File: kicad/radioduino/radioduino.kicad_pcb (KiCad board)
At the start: 2 copper layers, 130.5 x 70 mm, 48 parts, among them J1 Conn_01x03_Socket, J2 Conn_Coaxial_Small, J3 Conn_Coaxial_Small, J4 Conn_Coaxial_Small, J5 Conn_Coaxial_Small, J6 Conn_01x15, J7 Conn_01x15, Q1 SS8050, Q2 BSS138, Q3 BSS138, SW1 RotaryEncoder_Switch_MP, U1 PCF8574AT, U2 RT9193-33GB, Y1 Si5351A-B-GT

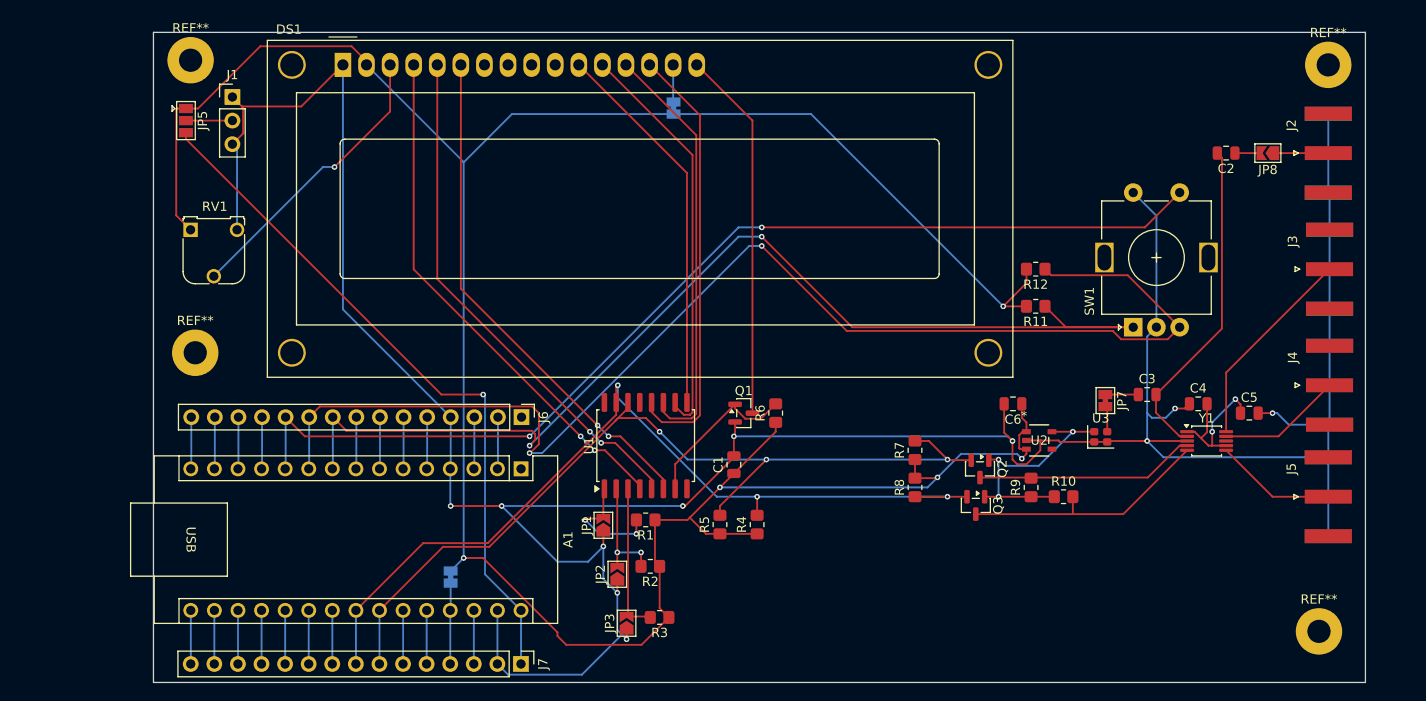
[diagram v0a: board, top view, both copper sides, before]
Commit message: pcb
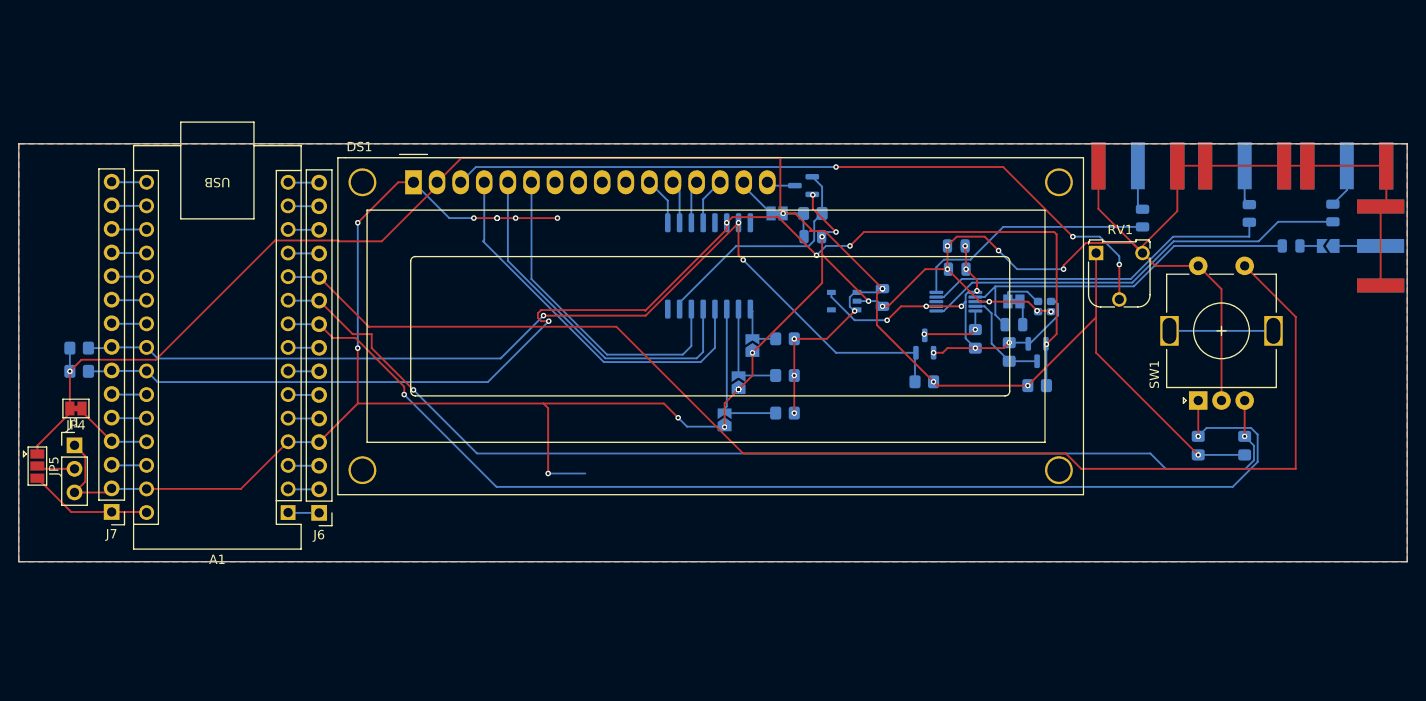
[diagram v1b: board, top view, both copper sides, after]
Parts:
- removed REF** (x4): MountingHole_2.5mm_Pad, MountingHole:MountingHole_2.5mm_Pad
- added C7: 100n, Capacitor_SMD:C_0805_2012Metric, B.Cu at (191.0, 65.0)
- added C8: 100n, Capacitor_SMD:C_0805_2012Metric, B.Cu at (202.5, 64.5)
- added C9: 100n, Capacitor_SMD:C_0805_2012Metric, B.Cu at (211.5, 64.5)
- C1, C2, C3, C4, C5, C6, J2, J3, J4, J5, JP1, JP2, JP3, JP7, JP8, Q1, Q2, Q3, R1, R10, R11, R12, R2, R3, R4, R5, R6, R7, R8, R9, U1, U2, U3, Y1: moved to B.Cu
- JP4: moved to F.Cu
- moved RV1 97.5 mm to (186.0, 68.8)
- moved R4 75.4 mm to (76.5, 79.0), turned to 0 degrees
- moved R5 70.9 mm to (76.5, 81.5), turned to 0 degrees
- moved J7 47.0 mm to (80.0, 96.6), turned to 180 degrees
- moved JP4 44.2 mm to (76.2, 85.5), turned to 180 degrees
- moved J1 41.2 mm to (76.0, 89.5)
- moved JP5 40.5 mm to (72.0, 91.7)
- moved C5 36.3 mm to (170.9, 68.0), turned to 180 degrees
- moved J5 35.7 mm to (213.0, 59.4), turned to 90 degrees
- moved Y1 30.9 mm to (170.9, 74.0), turned to 180 degrees
- moved C4 29.7 mm to (171.1, 70.5)
- moved R12 29.4 mm to (202.0, 89.5), turned to -90 degrees
- moved C1 26.0 mm to (155.5, 67.0), turned to 0 degrees
- moved R3 25.8 mm to (152.5, 86.0)
- moved U2 25.8 mm to (158.9, 73.9), turned to 180 degrees
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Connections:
- Y1 pad 10: Net-(J3-In) -> Net-(Y1-CLK0)
- Y1 pad 6: Net-(J5-In) -> Net-(Y1-CLK2)
- Y1 pad 9: Net-(J4-In) -> Net-(Y1-CLK1)
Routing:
- net +5V: track 284.5 -> 210.8 mm, vias 5 -> 11
- net /vin: track 74.4 -> 13.3 mm, vias 1 -> 0
- net Net-(DS1-VO): track 31.3 -> 80.2 mm, vias 1 -> 3
- net Net-(Y1-CLK2): track 0.00 -> 46.7 mm
- net Net-(DS1-D7): track 47.0 -> 5.12 mm
- net Net-(DS1-D6): track 45.8 -> 4.59 mm
- net /scl: track 94.4 -> 134.9 mm, vias 3 -> 5
- net Net-(DS1-D5): track 44.2 -> 4.65 mm
- net Net-(Y1-CLK1): track 0.00 -> 37.9 mm
- net Net-(DS1-LED(-)): track 40.0 -> 3.11 mm
- net Net-(DS1-D4): track 41.2 -> 5.18 mm
- net /d8: track 113.6 -> 141.2 mm, vias 2 -> 0
- net Net-(Y1-CLK0): track 0.00 -> 26.7 mm
- net GND: track 334.1 -> 310.5 mm, vias 11 -> 26
- net Net-(DS1-E): track 55.4 -> 35.4 mm, vias 2 -> 0
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- added copper zone on B.Cu, net GND
- added copper zone on F.Cu, net GND
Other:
- board size 130.5 x 70 mm -> 149.5 x 45 mm
